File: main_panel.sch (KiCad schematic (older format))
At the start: 18 parts

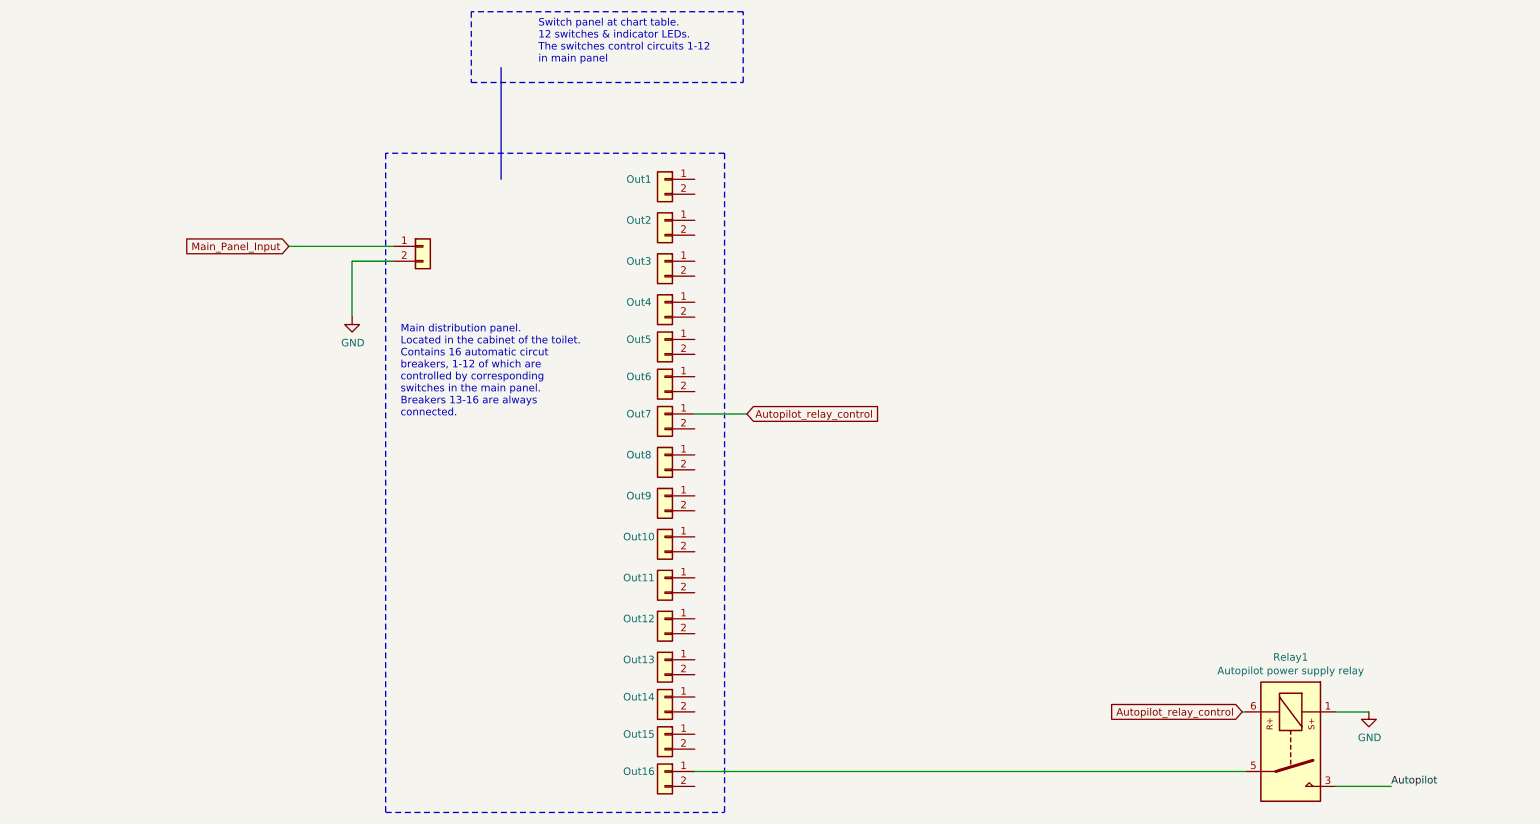
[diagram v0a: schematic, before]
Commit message: Several updates, maybe final version for season 2021
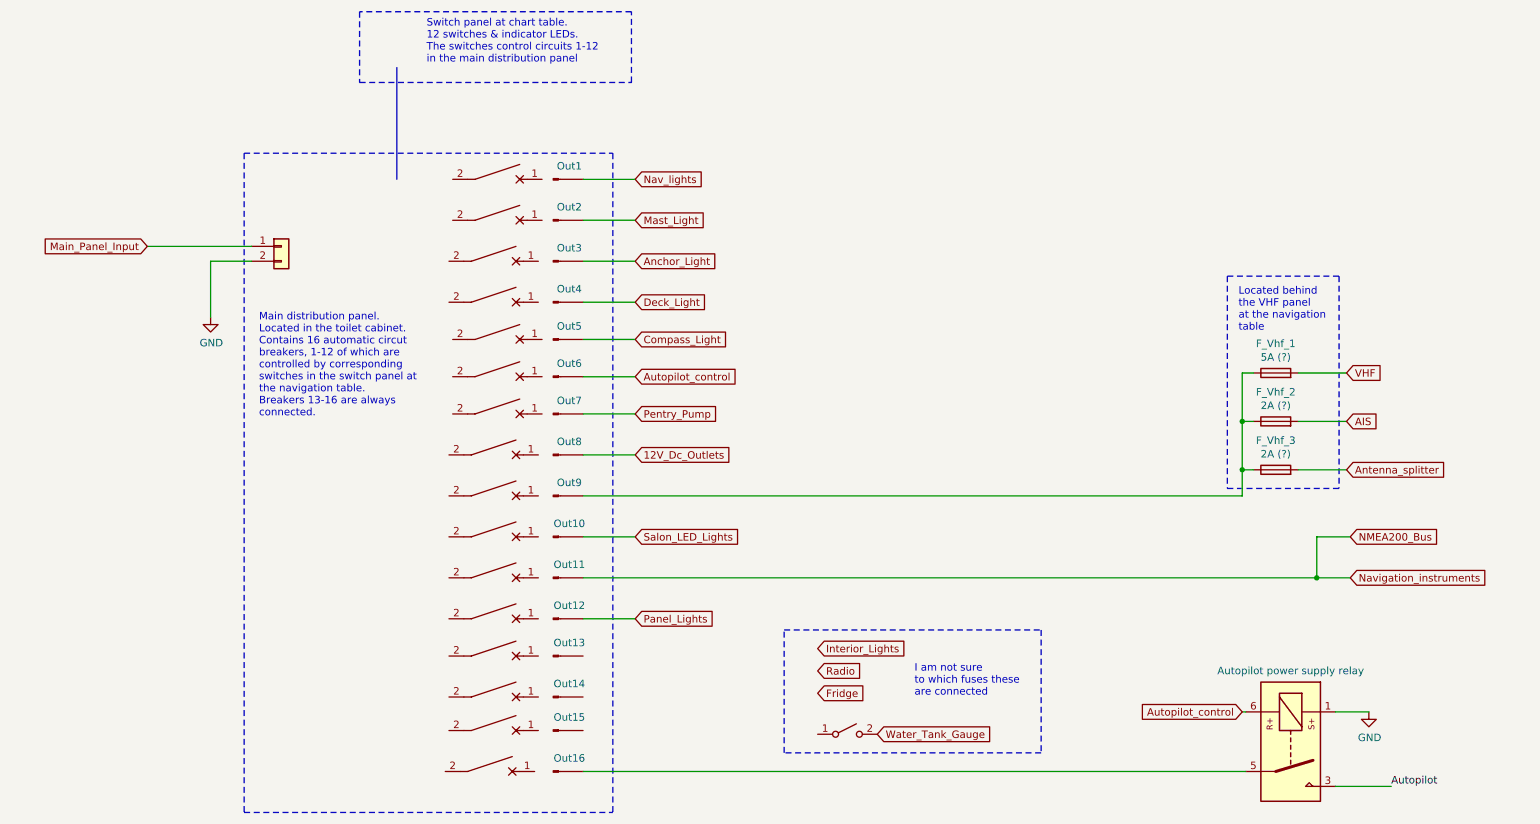
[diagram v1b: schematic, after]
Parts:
- removed Out1, Out10, Out11, Out12, Out13, Out14, Out15, Out16, Out2, Out3, Out4, Out5, Out6, Out7, Out8, Out9: Conn_01x02, symbol Connector_Generic:Conn_01x02
- added CB? (x16): 10A, symbol Device:CircuitBreaker_1P
- added F_Vhf_1: 5A (?), symbol Device:Fuse
- added F_Vhf_2, F_Vhf_3: 2A (?), symbol Device:Fuse
- added Out1, Out10, Out11, Out12, Out13, Out14, Out15, Out16, Out2, Out3, Out4, Out5, Out6, Out7, Out8, Out9: Conn_pin, symbol Simple_connector:Conn_pin
- added SW_tank_gauge: SW_SPST, symbol Switch:SW_SPST
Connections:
- net at Relay1.5: now also Out16.1 (Pin_1)
- net Autopilot_relay_control renamed Autopilot_control
- net Autopilot_control: now also Out6.1 (Pin_1)
- new net: F_Vhf_1.1, F_Vhf_2.1, F_Vhf_3.1, Out9.1 (Pin_1)
- new net 12V_Dc_Outlets: Out8.1 (Pin_1)
- new net AIS: F_Vhf_2.2
- new net Anchor_Light: Out3.1 (Pin_1)
- new net Antenna_splitter: F_Vhf_3.2
- new net Compass_Light: Out5.1 (Pin_1)
- new net Deck_Light: Out4.1 (Pin_1)
- new net Mast_Light: Out2.1 (Pin_1)
- new net NMEA200_Bus: Out11.1 (Pin_1)
- new net Nav_lights: Out1.1 (Pin_1)
- new net Panel_Lights: Out12.1 (Pin_1)
- new net Pentry_Pump: Out7.1 (Pin_1)
- new net Salon_LED_Lights: Out10.1 (Pin_1)
- new net VHF: F_Vhf_1.2
- new net Water_Tank_Gauge: SW_tank_gauge.2 (B)
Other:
- note added: "I am not sure\nto which fuses these \nare connected"
- note added: "Located behind \nthe VHF panel\nat the navigation \ntable"
- note added: "Main distribution panel. \nLocated in the toilet cabinet.\nContains 16 automatic circut\nbreakers, 1-12 of which are \ncontrolled by corresponding \nswitches in the switch panel at \nthe navigation table.\nBreakers 13-16 are always \nconnected."
- note added: "Switch panel at chart table. \n12 switches & indicator LEDs.\nThe switches control circuits 1-12\nin the main distribution panel"
- note removed: "Main distribution panel. \nLocated in the cabinet of the toilet.\nContains 16 automatic circut\nbreakers, 1-12 of which are \ncontrolled by corresponding \nswitches in the main panel.\nBreakers 13-16 are always \nconnected."
- note removed: "Switch panel at chart table. \n12 switches & indicator LEDs.\nThe switches control circuits 1-12\nin main panel"
